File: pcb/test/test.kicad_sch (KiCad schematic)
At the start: 16 parts, among them IC1 ADG904BRUZ-REEL7, J1 CONSMA013.062-G, J3 Conn_01x04, U2 TL081

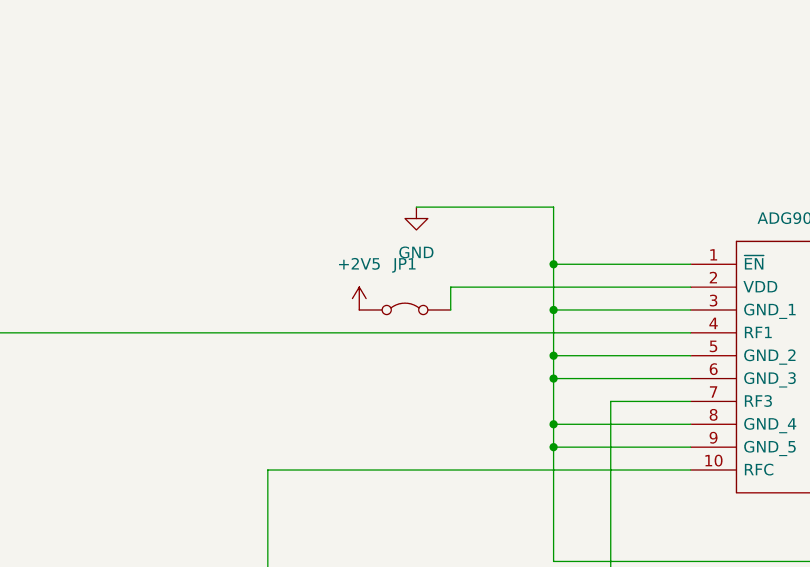
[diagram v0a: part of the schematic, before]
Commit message: ajustement pour impression
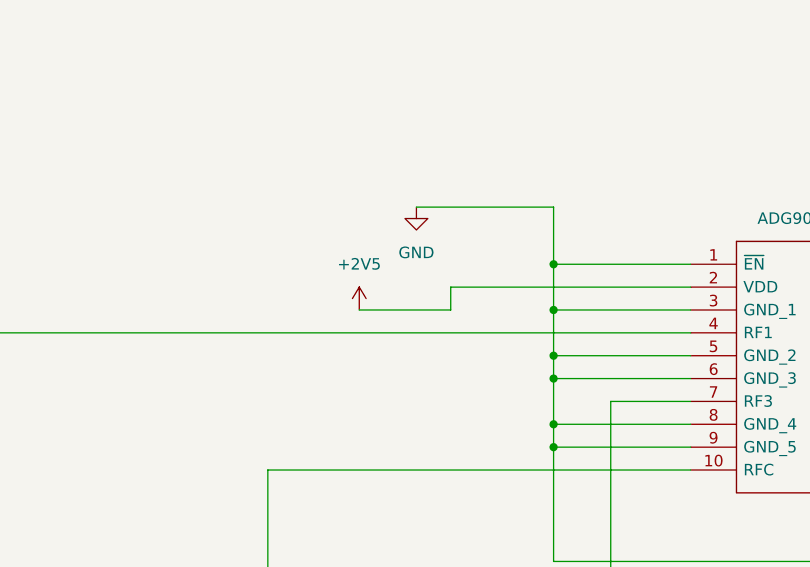
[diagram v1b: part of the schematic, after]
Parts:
- removed JP1: Jumper_2_Bridged, test_footprint_library:jumper20, symbol Jumper:Jumper_2_Bridged
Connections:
- net +2V5: now also IC1.2 (VDD)
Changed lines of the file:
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@@
+	(wire
+		(pts
+			(xy 71.12 128.27) (xy 81.28 128.27)
+		)
+		(stroke
+			(width 0)
+			(type default)
+		)
+	)
 	(wire
 		(pts
@@
 					(unit 1)
 				)
-			)
-		)
-	)
-	(symbol
-		(lib_id "Jumper:Jumper_2_Bridged")
-		(at 76.2 128.27 0)
-		(unit 1)
-		(exclude_from_sim yes)
-		(in_bom yes)
-		(on_board yes)
-		(dnp no)
-		(fields_autoplaced yes)
-		(property "Reference" "JP1"
-			(at 76.2 123.19 0)
-			(effects
-				(font
-					(size 1.27 1.27)
-				)
-			)
-		)
-		(property "Value" "Jumper_2_Bridged"
-			(at 76.2 125.73 0)
-			(effects
-				(font
-					(size 1.27 1.27)
-				)
-				(hide yes)
-			)
-		)
-		(property "Footprint" "test_footprint_library:jumper20"
-			(at 76.2 128.27 0)
-			(effects
-				(font
-					(size 1.27 1.27)
-				)
-				(hide yes)
-			)
-		)
-		(property "Datasheet" "~"
-			(at 76.2 128.27 0)
-			(effects
-				(font
-					(size 1.27 1.27)
-				)
-				(hide yes)
-			)
-		)
-		(property "Description" "Jumper, 2-pole, closed/bridged"
-			(at 76.2 128.27 0)
-			(effects
-				(font
-					(size 1.27 1.27)
-				)
-				(hide yes)
-			)
-		)
-		(pin "2"
-		)
-		(pin "1"
-		)
-		(instances
-			(project ""
-				(path "/bb1015a8-5dcf-444f-b1dc-3665f721c6b4"
-					(reference "JP1")
-					(unit 1)
-				)
